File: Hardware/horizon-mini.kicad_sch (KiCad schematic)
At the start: 73 parts, among them J2 Conn_01x02_Pin, J3 Micro_SD_Card_Det1, J7 USB_C_Receptacle_USB2.0_16P, J8 Conn_02x03_Counter_Clockwise, Q1 BSS138, Q10 DMG2301L, U1 TPS82130, U16 AP2112K-3.3, U2 TPS61092, U3 LTC4412xS6, U4 TMCU, U6 NAND, U7 LPS22HB, U9 LSM6DS3

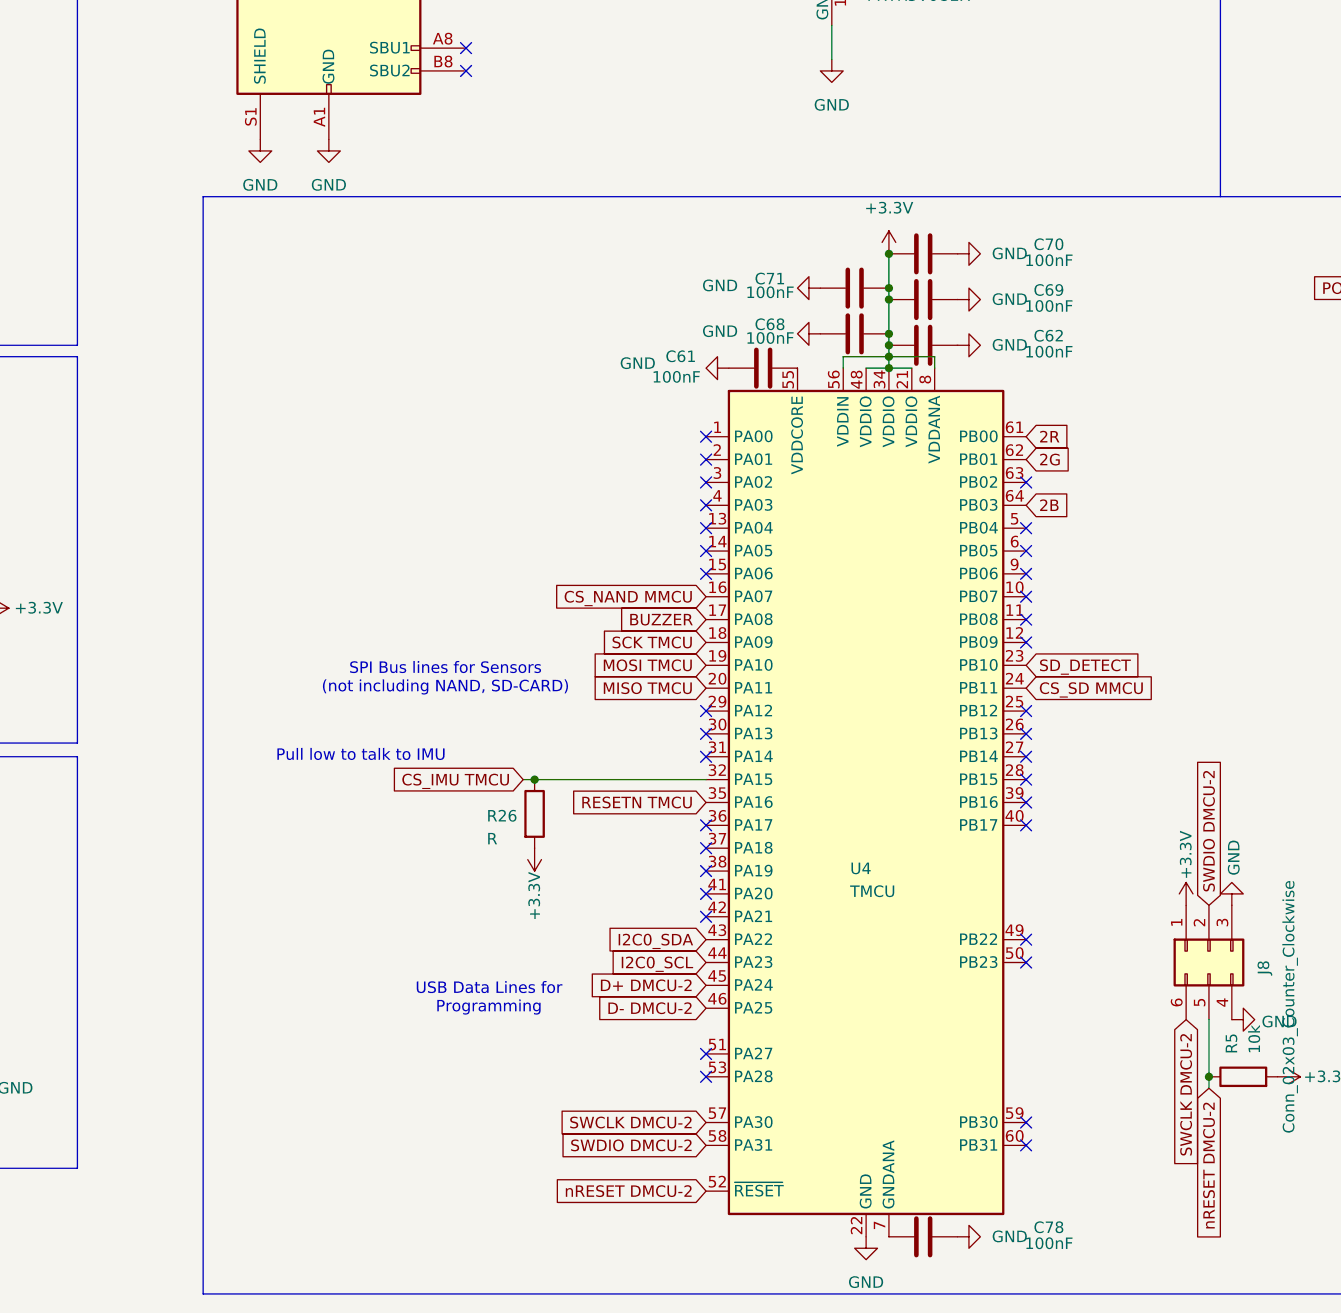
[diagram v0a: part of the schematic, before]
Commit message: uuuh, fixed shematic and re-did most of the routing for the new MCU :(
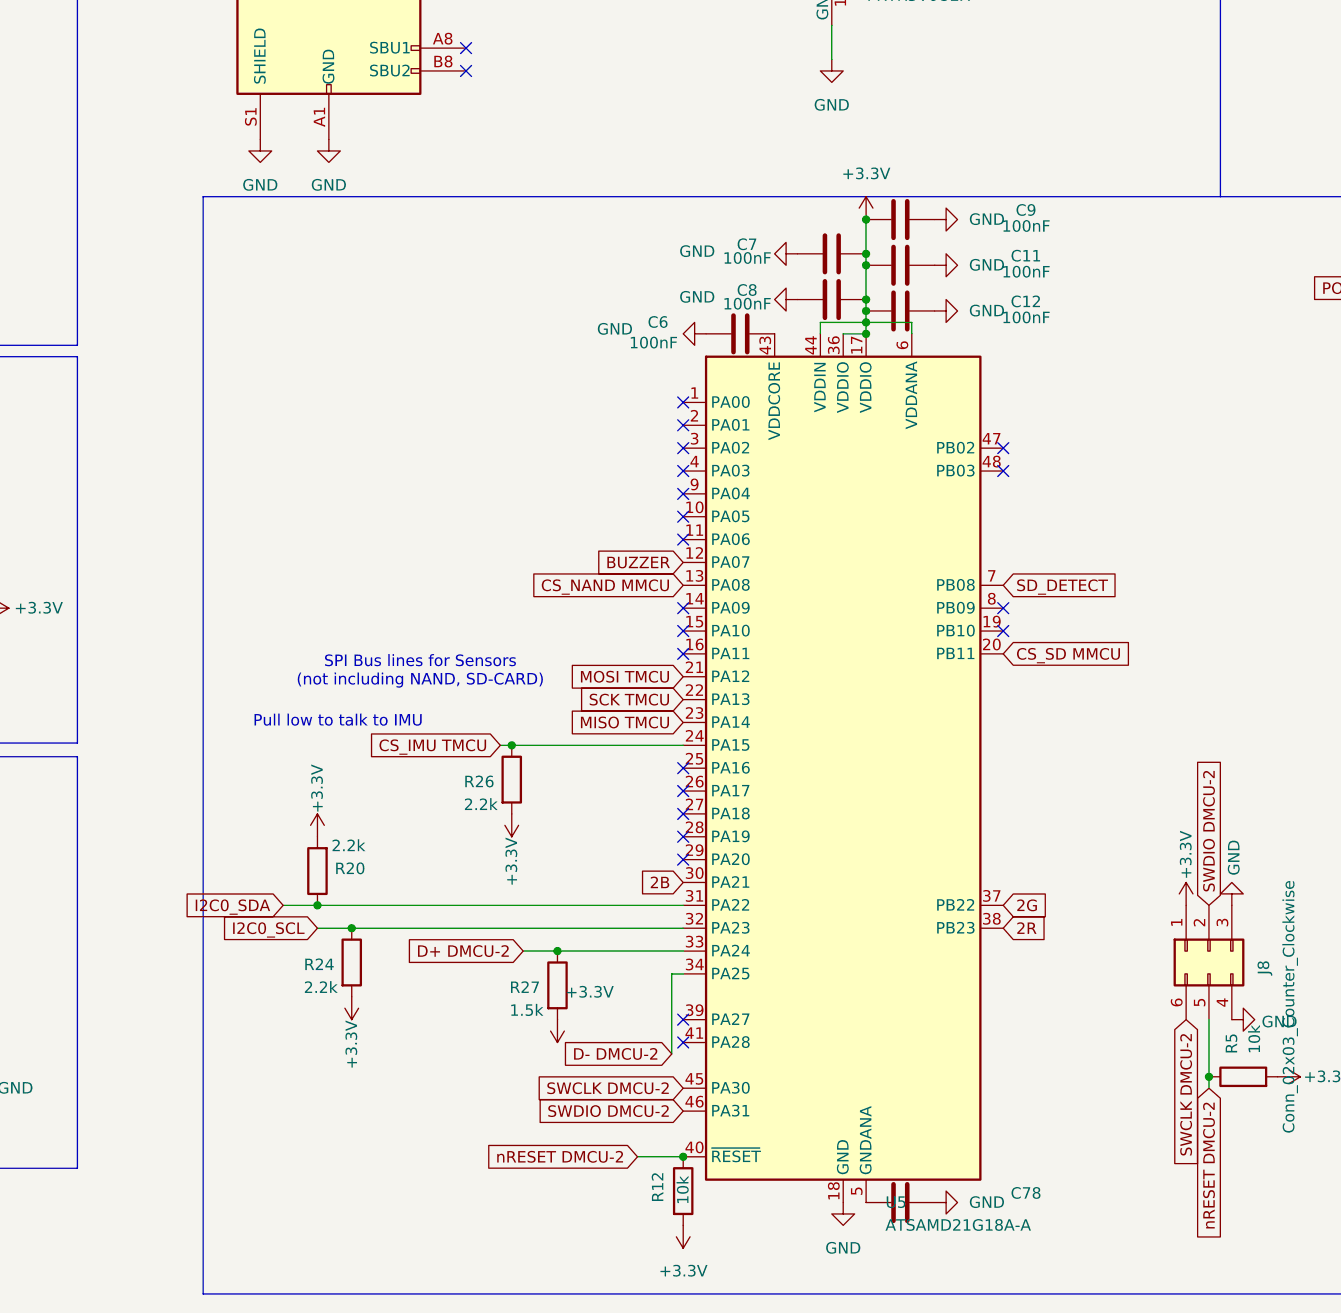
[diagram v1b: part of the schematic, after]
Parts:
- removed C61, C62, C68, C69, C70, C71: 100nF, Capacitor_SMD:C_0603_1608Metric, symbol Device:C
- removed U4: TMCU, Package_QFP:TQFP-64_10x10mm_P0.5mm, symbol MCU_Microchip_SAMD:ATSAMD21J16B-A
- added C11, C12, C6, C7, C8, C9: 100nF, Capacitor_SMD:C_0603_1608Metric, symbol Device:C
- added R12: 10k, Resistor_SMD:R_0603_1608Metric, symbol Device:R
- added R20, R24: 2.2k, Resistor_SMD:R_0603_1608Metric, symbol Device:R
- added R27: 1.5k, Resistor_SMD:R_0603_1608Metric, symbol Device:R
- added U5: ATSAMD21G18A-A, Package_QFP:TQFP-48_7x7mm_P0.5mm, symbol MCU_Microchip_SAMD:ATSAMD21G18A-A
- R26: value R -> 2.2k
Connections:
- net +3.3V: now also C11.2, C12.2, C7.2, C8.2, C9.2, R12.2, R20.2, R24.2, R27.2, U5.17 (VDDIO), U5.36 (VDDIO), U5.44 (VDDIN), U5.6 (VDDANA)
- net 2B: now also U5.30 (PA21)
- net 2G: now also U5.37 (PB22)
- net 2R: now also U5.38 (PB23)
- net BUZZER: now also U5.12 (PA07)
- net CS_IMU TMCU: now also U5.24 (PA15)
- net CS_NAND MMCU: now also U5.13 (PA08)
- net CS_SD MMCU: now also U5.20 (PB11)
- net D+ DMCU-2: now also R27.1, U5.33 (PA24)
- net D- DMCU-2: now also U5.34 (PA25)
- net GND: now also C11.1, C12.1, C6.1, C7.1, C8.1, C9.1, U5.18 (GND), U5.35 (GND), U5.42 (GND)
- net I2C0_SCL: now also R24.1, U5.32 (PA23)
- net I2C0_SDA: now also R20.1, U5.31 (PA22)
- net MISO TMCU: now also U5.23 (PA14)
- net MOSI TMCU: now also U5.21 (PA12)
- net SCK TMCU: now also U5.22 (PA13)
- net SD_DETECT: now also U5.7 (PB08)
- net SWCLK DMCU-2: now also U5.45 (PA30)
- net SWDIO DMCU-2: now also U5.46 (PA31)
- net nRESET DMCU-2: now also R12.1, U5.40 (~{RESET})
- net at C78.2: now also U5.5 (GNDANA)
- new net: C6.2, U5.43 (VDDCORE)
- no-connect marks 42 -> 29
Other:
- note removed: "USB Data Lines for Programming"
- moved on the sheet: C78, R26

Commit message: Revert "Merge branch 'main' of https://github.com/Horizon-Avionics/Horizon-Mini"
This reverts commit 9a022c3cd95984122db224f561db0d5bee869fb2, reversing
changes made to 44f91161868ebb609577ad71ea77d3c9bc8dd4bf.
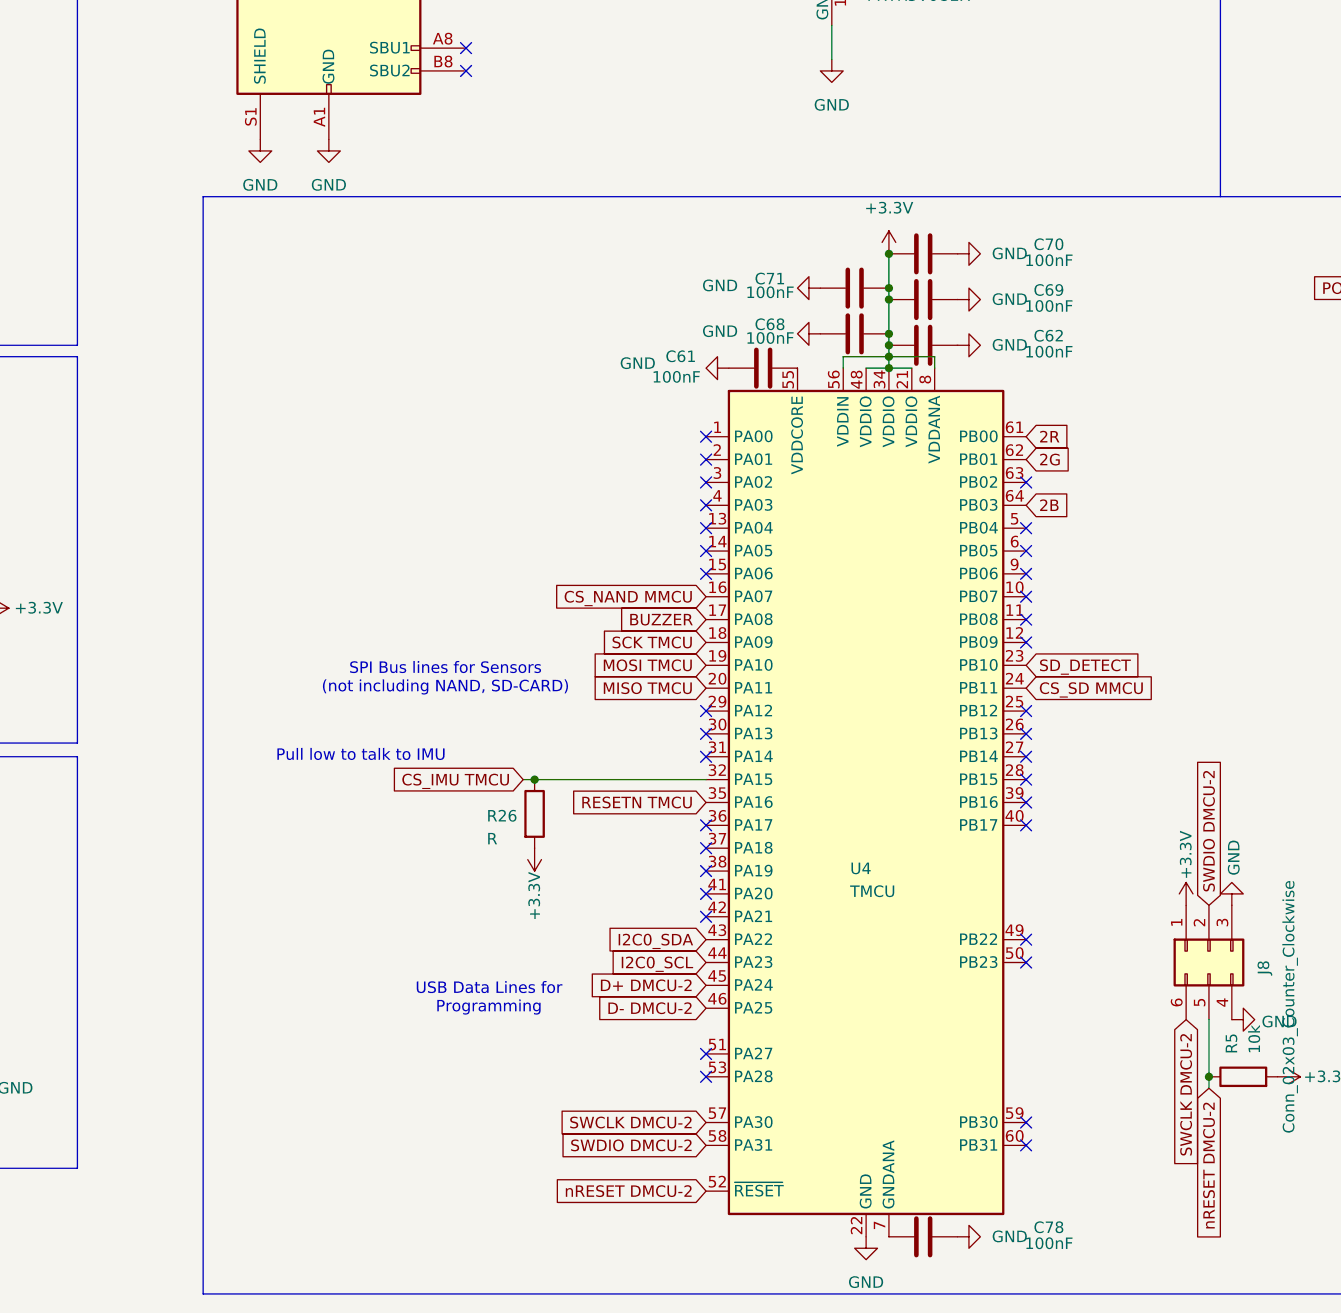
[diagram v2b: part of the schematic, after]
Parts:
- removed C11, C12, C6, C7, C8, C9: 100nF, Capacitor_SMD:C_0603_1608Metric, symbol Device:C
- removed R12: 10k, Resistor_SMD:R_0603_1608Metric, symbol Device:R
- removed R20, R24: 2.2k, Resistor_SMD:R_0603_1608Metric, symbol Device:R
- removed R27: 1.5k, Resistor_SMD:R_0603_1608Metric, symbol Device:R
- removed U5: ATSAMD21G18A-A, Package_QFP:TQFP-48_7x7mm_P0.5mm, symbol MCU_Microchip_SAMD:ATSAMD21G18A-A
- added C61, C62, C68, C69, C70, C71: 100nF, Capacitor_SMD:C_0603_1608Metric, symbol Device:C
- added U4: TMCU, Package_QFP:TQFP-64_10x10mm_P0.5mm, symbol MCU_Microchip_SAMD:ATSAMD21J16B-A
- R26: value 2.2k -> R
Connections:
- net +3.3V: now also C62.2, C68.2, C69.2, C70.2, C71.2, U4.21 (VDDIO), U4.34 (VDDIO), U4.48 (VDDIO), U4.56 (VDDIN), U4.8 (VDDANA)
- net 2B: now also U4.64 (PB03)
- net 2G: now also U4.62 (PB01)
- net 2R: now also U4.61 (PB00)
- net BUZZER: now also U4.17 (PA08)
- net CS_IMU TMCU: now also U4.32 (PA15)
- net CS_NAND MMCU: now also U4.16 (PA07)
- net CS_SD MMCU: now also U4.24 (PB11)
- net D+ DMCU-2: now also U4.45 (PA24)
- net D- DMCU-2: now also U4.46 (PA25)
- net GND: now also C61.1, C62.1, C68.1, C69.1, C70.1, C71.1, U4.22 (GND), U4.33 (GND), U4.47 (GND), U4.54 (GND)
- net I2C0_SCL: now also U4.44 (PA23)
- net I2C0_SDA: now also U4.43 (PA22)
- net MISO TMCU: now also U4.20 (PA11)
- net MOSI TMCU: now also U4.19 (PA10)
- net SCK TMCU: now also U4.18 (PA09)
- net SD_DETECT: now also U4.23 (PB10)
- net SWCLK DMCU-2: now also U4.57 (PA30)
- net SWDIO DMCU-2: now also U4.58 (PA31)
- net nRESET DMCU-2: now also U4.52 (~{RESET})
- net at C78.2: now also U4.7 (GNDANA)
- new net: C61.2, U4.55 (VDDCORE)
- new net RESETN TMCU: U4.35 (PA16)
- no-connect marks 29 -> 42
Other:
- note added: "USB Data Lines for Programming"
- moved on the sheet: C78, R26
